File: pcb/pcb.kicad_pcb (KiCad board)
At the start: 2 copper layers, 43.2 x 33 mm, 7 parts, among them U1 xiao-ble

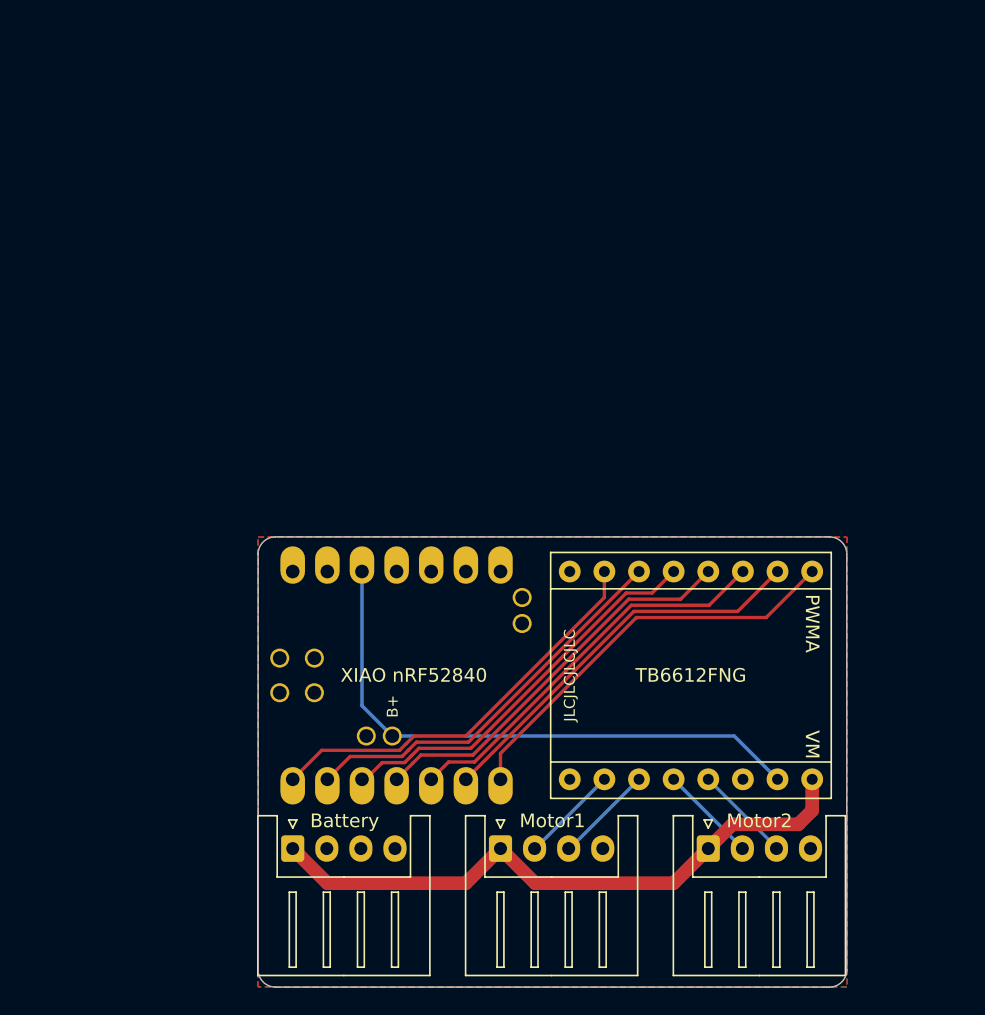
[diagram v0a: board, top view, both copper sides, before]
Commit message: v2
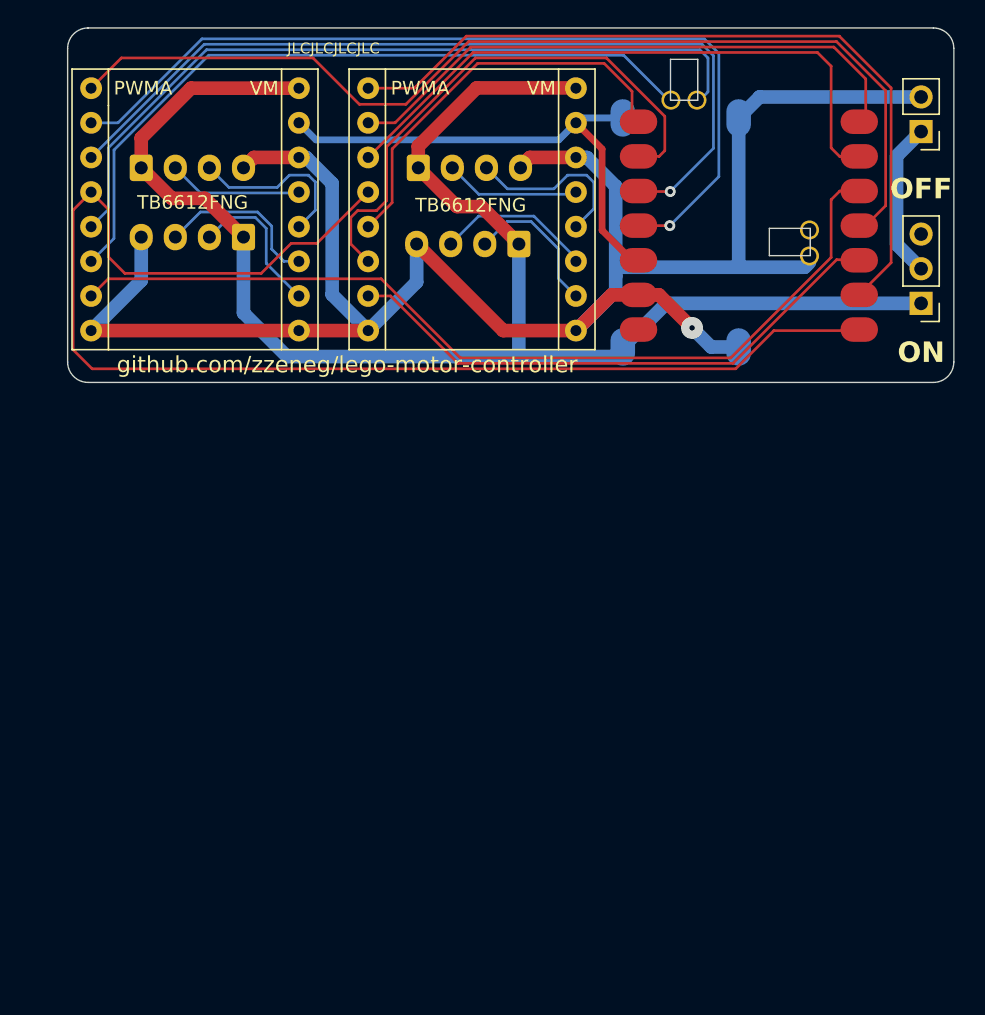
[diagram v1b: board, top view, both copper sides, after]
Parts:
- removed Battery: Conn_01x04_Female, Connector_JST:JST_XH_S4B-XH-A_1x04_P2.50mm_Horizontal
- removed G***: LOGO, lego:logo
- removed G***: LOGO, lego:seeed-logo
- added J1: Conn_01x02_Socket, Connector_PinHeader_2.54mm:PinHeader_1x02_P2.54mm_Vertical, F.Cu at (155.3, 41.4)
- added J2: Conn_01x04_Socket, lego:voltage-converter, B.Cu at (137.7, 48.8)
- added Motor3: Conn_01x04_Female, Connector_JST:JST_XH_S4B-XH-A_1x04_P2.50mm_Horizontal, B.Cu at (98.1, 44.1)
- added Motor4: Conn_01x04_Female, Connector_JST:JST_XH_S4B-XH-A_1x04_P2.50mm_Horizontal, B.Cu at (105.6, 49.1)
- added SW1: SW_SPDT, Connector_PinHeader_2.54mm:PinHeader_1x03_P2.54mm_Vertical, F.Cu at (155.3, 54.0)
- added TB2: TB6612_Breakout, lego:TB6612-breakout, F.Cu at (94.4, 38.2)
- Motor1, Motor2: moved to B.Cu
- TB1: footprint lego:Breakout-16_17.8x20.3mm -> lego:TB6612-breakout
- U1: value xiao-ble -> MCU_xiao-ble; footprint lego:xiao-ble-tht -> zzkeeb:MCU_xiao-ble-smd
- moved U1 52.6 mm to (142.7, 48.3), turned to 180 degrees
- moved Motor1 50.3 mm to (118.4, 44.1)
- moved TB1 48.1 mm to (114.8, 38.2), turned to 0 degrees
- moved Motor2 46.5 mm to (125.8, 49.6), turned to 180 degrees
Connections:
- Motor1 pad 2: B01 -> A01_1
- Motor1 pad 3: B02 -> A02_1
- Motor2 pad 2: A02 -> B01_1
- Motor2 pad 3: A01 -> B02_1
- TB1 pad 1: PWMA -> PWMA_1
- TB1 pad 10: B01 -> B01_1
- TB1 pad 11: B02 -> B02_1
- TB1 pad 12: A02 -> A02_1
- TB1 pad 13: A01 -> A01_1
- TB1 pad 2: AIN2 -> AIN2_1
- TB1 pad 3: AIN1 -> AIN1_1
- TB1 pad 5: BIN1 -> BIN1_1
- TB1 pad 6: BIN2 -> BIN2_1
- TB1 pad 7: PWMB -> PWMB_1
- U1 pad 1: PWMB -> STBY
- U1 pad 10: unconnected-(U1-Pad10) -> AIN1_2
- U1 pad 11: unconnected-(U1-Pad11) -> AIN2_2
- U1 pad 19: +3.3V -> unconnected-(U1-BAT-Pad19)
- U1 pad 2: BIN2 -> PWMA_1
- U1 pad 21: unconnected-(U1-Pad21) -> BIN1_2
- U1 pad 22: unconnected-(U1-Pad22) -> BIN2_2
- U1 pad 3: BIN1 -> PWMB_1
- U1 pad 4: STBY -> PWMA_2
- U1 pad 5: AIN1 -> PWMB_2
- U1 pad 6: AIN2 -> AIN1_1
- U1 pad 7: PWMA -> AIN2_1
- U1 pad 8: unconnected-(U1-Pad8) -> BIN1_1
- U1 pad 9: unconnected-(U1-Pad9) -> BIN2_1
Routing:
- net GND: track 0.00 -> 144.1 mm, vias 0 -> 1
- net PWMA_2: track 0.00 -> 74.5 mm
- net +9V: track 45.8 -> 116.0 mm
- net STBY: track 29.2 -> 99.3 mm
- net PWMB_2: track 0.00 -> 67.3 mm
- net AIN2_2: track 0.00 -> 65.9 mm, vias 0 -> 1
- net AIN1_2: track 0.00 -> 63.5 mm, vias 0 -> 1
- net BIN1_2: track 0.00 -> 57.0 mm
- net PWMA_1: track 0.00 -> 57.0 mm
- net BIN2_2: track 0.00 -> 53.9 mm
- net AIN1_1: track 0.00 -> 46.4 mm
- net AIN2_1: track 0.00 -> 42.9 mm
- net PWMB_1: track 0.00 -> 42.2 mm
- net BIN2_1: track 0.00 -> 40.8 mm
- net PWMB: track 30.3 -> 0.00 mm
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- removed copper zone on B.Cu, net GND
- removed copper zone on F.Cu, net GND
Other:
- board size 43.2 x 33 mm -> 65 x 26 mm
- board text added: "+"
- board text added: "-"
- board text added: "3.3V"
- board text added: "9V"
- board text added: "OFF"
- board text added: "ON"
- board text added: "github.com/zzeneg/lego-motor-controller"
- board text removed: "B+"
- board text removed: "XIAO nRF52840"
- board text removed: "https://github.com/zzeneg/lego-motor-controller"
